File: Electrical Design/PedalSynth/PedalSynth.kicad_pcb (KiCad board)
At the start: 2 copper layers, 71.9 x 39 mm, 27 parts, among them J1 AudioJack3, J3 Barrel_Jack, U1 TPA3136D2PWPR

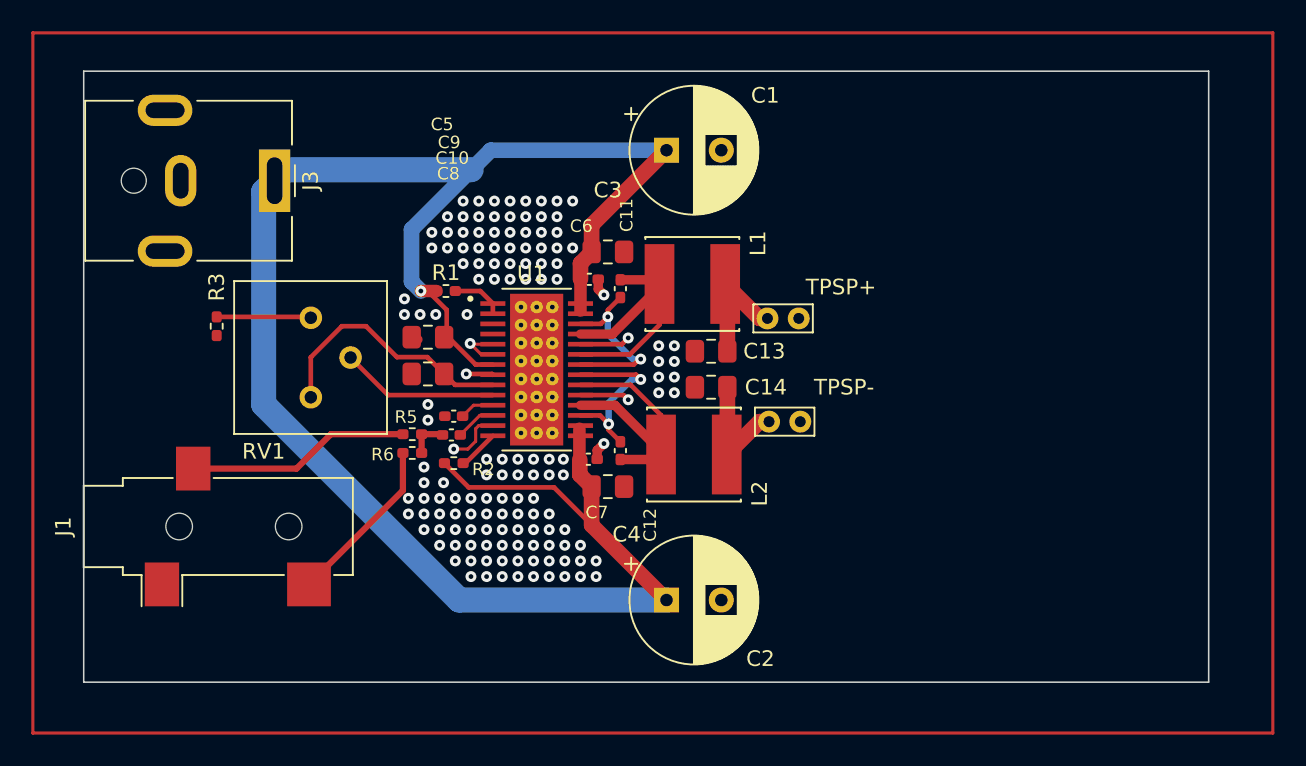
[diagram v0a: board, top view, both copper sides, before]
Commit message: r1.0 amp pcb
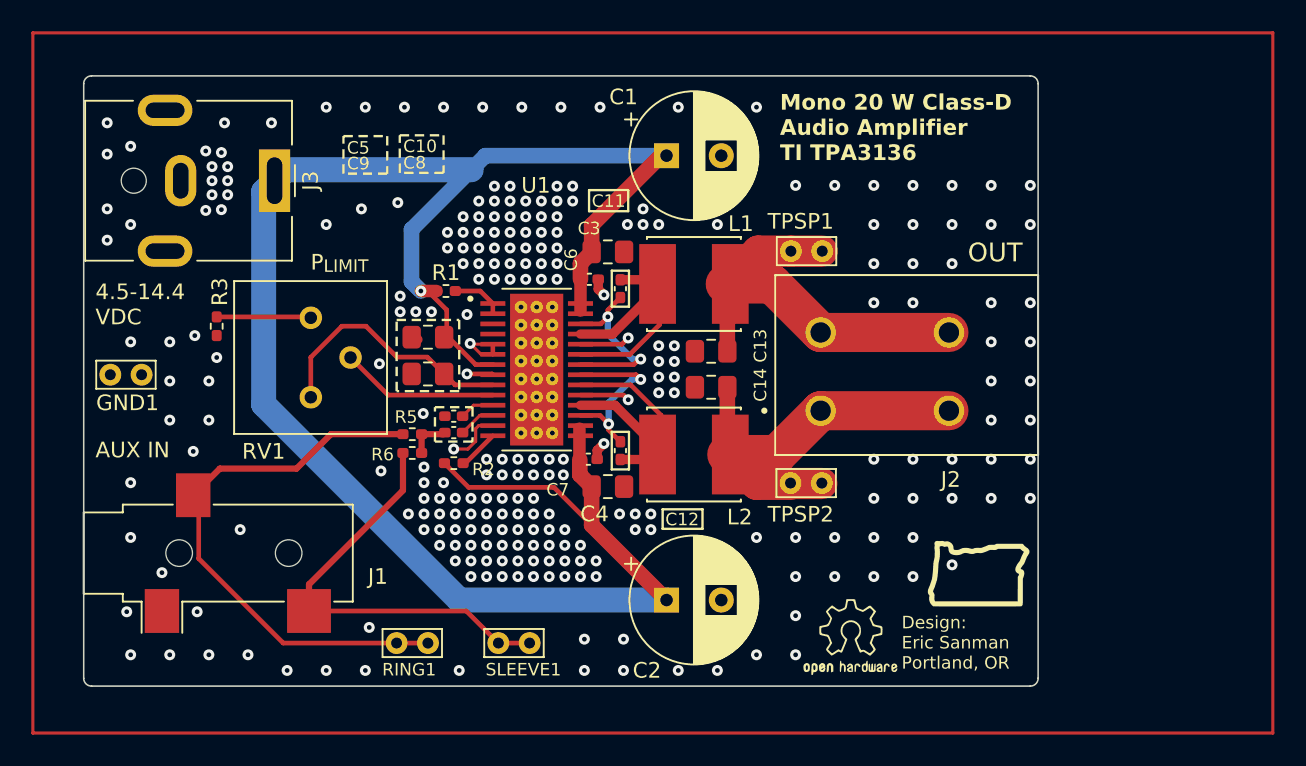
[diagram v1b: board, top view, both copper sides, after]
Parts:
- added G***: LOGO, LOGO, F.Cu at (181.3, 92.6)
- added G***: LOGO, LOGO, F.Cu at (173.1, 96.7)
- added GND1: TestPoint, TestPoint:TestPoint_Bridge_Pitch2.0mm_Drill0.7mm, F.Cu at (125.8, 79.9)
- added J2: Pheonix Latching Connector (1190297), Pheonix-2P-Level1190297:PHOENIX_1190297, F.Cu at (185.1, 85.0)
- added RING1: TestPoint, TestPoint:TestPoint_Bridge_Pitch2.0mm_Drill0.7mm, F.Cu at (144.1, 97.0)
- added SLEEVE1: TestPoint, TestPoint:TestPoint_Bridge_Pitch2.0mm_Drill0.7mm, F.Cu at (150.6, 97.0)
- moved TPSP1 4.55 mm to (169.3, 72.0)
- moved TPSP2 4.16 mm to (169.3, 86.8)
- moved J1 1.70 mm to (132.7, 91.3)
- moved C1 0.35 mm to (161.3, 65.9)
- moved C8 0.21 mm to (147.8, 83.6)
- moved L1 0.10 mm to (163.1, 74.1)
- renumbered TPSP+ to TPSP1, TPSP- to TPSP2
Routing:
- net Net-(J1-PadR): track 14.3 -> 36.1 mm
- net /SPK+: track 7.97 -> 27.0 mm
- net /SPK-: track 7.89 -> 26.6 mm
- net Net-(J1-PadT): track 10.9 -> 27.5 mm
- net GND: track 18.9 -> 19.5 mm, vias 143 -> 275
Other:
- board size 71.9 x 39 mm -> 61 x 39 mm
- board text added: "4.5-14.4 VDC"
- board text added: "AUX IN"
- board text added: "Design: Eric Sanman Portland, OR"
- board text added: "Mono 20 W Class-D Audio Amplifier TI TPA3136"
- board text added: "OUT"
- board text added: "P_{LIMIT}"
